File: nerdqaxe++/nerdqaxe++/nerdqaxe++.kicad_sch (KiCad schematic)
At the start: 9 parts, among them J1 XT30

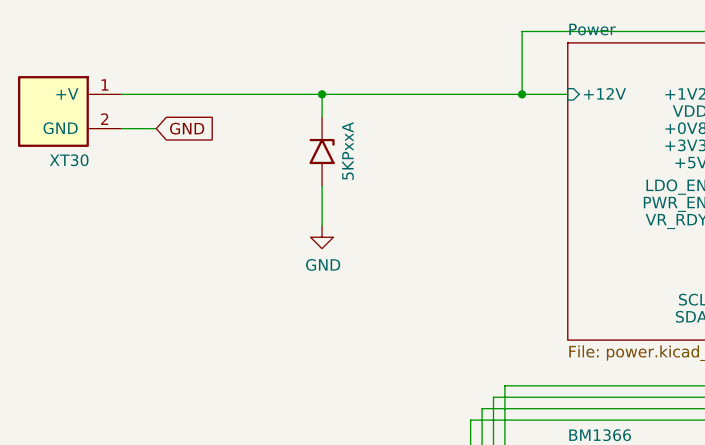
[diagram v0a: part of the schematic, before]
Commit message: Powermining revision
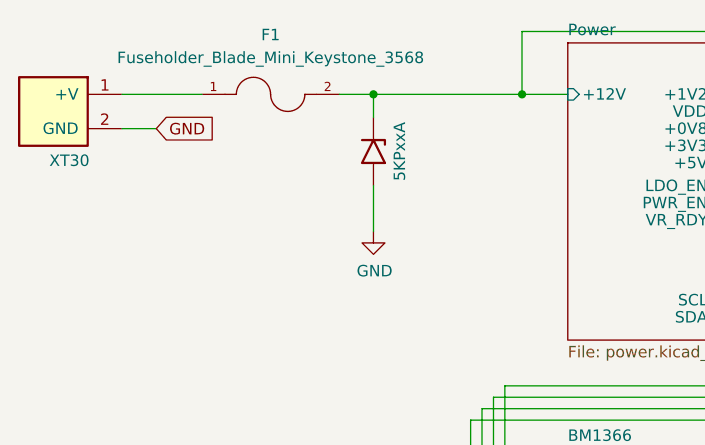
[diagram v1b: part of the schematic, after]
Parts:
- added F1: Fuseholder_Blade_Mini_Keystone_3568, 8Axe:Fuseholder Blade_3568, symbol Fuseholder Blade 3568:3568
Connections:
- net Power/+12V: now also F1.2; no longer J1.1 (+V)
- new net: F1.1, J1.1 (+V)
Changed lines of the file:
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@@
 	)
 	(junction
-		(at 55.245 52.07)
+		(at 60.96 52.07)
 		(diameter 0)
 		(color 0 0 0 0)
@@
 	(wire
 		(pts
-			(xy 33.02 52.07) (xy 55.245 52.07)
-		)
-		(stroke
-			(width 0)
-			(type default)
-		)
-	)
-	(wire
-		(pts
-			(xy 55.245 54.61) (xy 55.245 52.07)
+			(xy 60.96 54.61) (xy 60.96 52.07)
 		)
 		(stroke
@@
 	(wire
 		(pts
-			(xy 55.245 66.675) (xy 55.245 62.23)
+			(xy 60.96 62.23) (xy 60.96 67.31)
 		)
 		(stroke
@@
 	(wire
 		(pts
+			(xy 57.15 52.07) (xy 60.96 52.07)
+		)
+		(stroke
+			(width 0)
+			(type default)
+		)
+	)
+	(wire
+		(pts
 			(xy 99.695 57.785) (xy 114.3 57.785)
 		)
@@
 	(wire
 		(pts
+			(xy 33.02 52.07) (xy 41.91 52.07)
+		)
+		(stroke
+			(width 0)
+			(type default)
+		)
+	)
+	(wire
+		(pts
 			(xy 75.565 84.455) (xy 75.565 97.79)
 		)
@@
 	(wire
 		(pts
+			(xy 60.96 52.07) (xy 77.47 52.07)
+		)
+		(stroke
+			(width 0)
+			(type default)
+		)
+	)
+	(wire
+		(pts
 			(xy 99.695 55.88) (xy 113.03 55.88)
 		)
@@
 		(pts
 			(xy 123.19 66.04) (xy 123.19 94.615)
-		)
-		(stroke
-			(width 0)
-			(type default)
-		)
-	)
-	(wire
-		(pts
-			(xy 55.245 52.07) (xy 77.47 52.07)
 		)
 		(stroke
@@
 	(symbol
 		(lib_id "power:GND")
-		(at 55.245 66.675 0)
+		(at 60.96 67.31 0)
 		(unit 1)
 		(exclude_from_sim no)
@@
 		(dnp no)
 		(property "Reference" "#PWR04"
-			(at 55.245 73.025 0)
+			(at 60.96 73.66 0)
 			(effects
 				(font
@@
 		)
 		(property "Value" "GND"
-			(at 55.372 71.0692 0)
+			(at 61.087 71.7042 0)
 			(effects
 				(font
@@
 		)
 		(property "Footprint" ""
-			(at 55.245 66.675 0)
+			(at 60.96 67.31 0)
 			(effects
 				(font
@@
 		)
 		(property "Datasheet" ""
-			(at 55.245 66.675 0)
+			(at 60.96 67.31 0)
 			(effects
 				(font
@@
 		)
 		(property "Description" ""
-			(at 55.245 66.675 0)
+			(at 60.96 67.31 0)
 			(effects
 				(font
@@
 	(symbol
 		(lib_id "Diode:5KPxxA")
-		(at 55.245 58.42 270)
+		(at 60.96 58.42 270)
 		(unit 1)
 		(exclude_from_sim no)
@@
 		(dnp no)
 		(property "Reference" "D1"
-			(at 52.324 57.15 0)
+			(at 58.039 57.15 0)
 			(effects
 				(font
@@
 		)
 		(property "Value" "5KPxxA"
-			(at 58.166 58.42 0)
+			(at 63.881 58.42 0)
 			(effects
 				(font
@@
 		)
 		(property "Footprint" "Diode_SMD:D_SMB"
-			(at 50.165 58.42 0)
+			(at 55.88 58.42 0)
 			(effects
 				(font
@@
 		)
 		(property "Datasheet" "https://diotec.com/tl_files/diotec/files/pdf/datasheets/5kp65.pdf"
-			(at 55.245 57.15 0)
+			(at 60.96 57.15 0)
 			(effects
 				(font
@@
 		)
 		(property "Description" "5000W unidirectional Transient Voltage Suppressor, P-600"
-			(at 55.245 58.42 0)
+			(at 60.96 58.42 0)
 			(effects
 				(font
@@
 		)
 		(property "Distributor" "D"
-			(at 55.245 58.42 0)
+			(at 60.96 58.42 0)
 			(effects
 				(font
@@
 		)
 		(property "OrderNr" "SMBJ12ALFCT-ND"
-			(at 55.245 58.42 0)
+			(at 60.96 58.42 0)
 			(effects
 				(font
@@
 		)
 		(property "PARTNO" "SMBJ12A"
-			(at 55.245 58.42 0)
+			(at 60.96 58.42 0)
 			(effects
 				(font
@@
 		)
 		(property "Manufacturer " "UMW(Youtai Semiconductor Co., Ltd.)"
-			(at 55.245 58.42 0)
+			(at 60.96 58.42 0)
 			(effects
 				(font
@@
 		)
 		(property "LCSC" "C3001973"
-			(at 55.245 58.42 0)
+			(at 60.96 58.42 0)
 			(effects
 				(font
@@
 					(unit 1)
 				)
+			)
+		)
+	)
+	(symbol
+		(lib_id "Fuseholder Blade 3568:3568")
+		(at 49.53 52.07 0)
+		(unit 1)
+		(exclude_from_sim no)
+		(in_bom yes)
+		(on_board yes)
+		(dnp no)
+		(fields_autoplaced yes)
+		(property "Reference" "F1"
+			(at 49.53 45.466 0)
+			(effects
+				(font
+					(size 1.27 1.27)
+				)
+			)
+		)
+		(property "Value" "Fuseholder_Blade_Mini_Keystone_3568"
+			(at 49.53 48.006 0)
+			(effects
+				(font
+					(size 1.27 1.27)
+				)
+			)
+		)
+		(property "Footprint" "8Axe:Fuseholder Blade_3568"
+			(at 49.53 52.07 0)
+			(effects
+				(font
+					(size 1.27 1.27)
+				)
+				(justify bottom)
+				(hide yes)
+			)
+		)
+		(property "Datasheet" ""
+			(at 49.53 52.07 0)
+			(effects
+				(font
+					(size 1.27 1.27)
+				)
+				(hide yes)
+			)
+		)
+		(property "Description" "Fuseholder Mini Blade"
+			(at 49.53 52.07 0)
+			(effects
+				(font
+					(size 1.27 1.27)
+				)
+				(hide yes)
+			)
+		)
+		(property "Manufacturer" "3568"
+			(at 49.53 52.07 0)
+			(effects
+				(font
+					(size 1.27 1.27)
+				)
+				(justify bottom)
+				(hide yes)
+			)
+		)
+		(property "Distributor" "D"
+			(at 49.53 52.07 0)
+			(effects
+				(font
+					(size 1.27 1.27)
+				)
+				(hide yes)
+			)
+		)
+		(property "OrderNr" "36-3568-ND"
+			(at 49.53 52.07 0)
+			(effects
+				(font
+					(size 1.27 1.27)
+				)
+				(hide yes)
+			)
+		)
+		(pin "1"
+		)
+		(pin "2"
+		)
+		(instances
+			(project "nerdqaxe++"
+				(path "/e63e39d7-6ac0-4ffd-8aa3-1841a4541b55"
+					(reference "F1")
+					(unit 1)
+				)
